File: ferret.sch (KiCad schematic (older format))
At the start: 0 parts

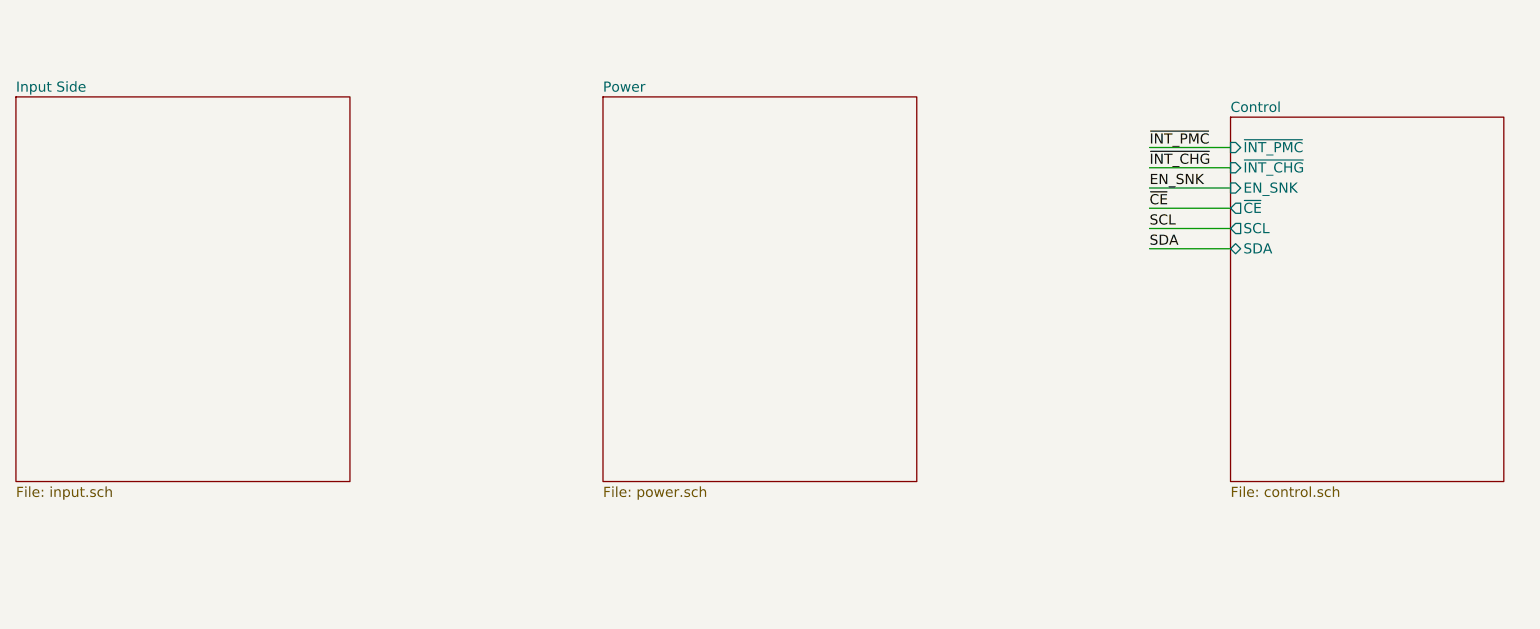
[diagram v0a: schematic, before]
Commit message: I'm pretty happy with it now, will place tomorrow
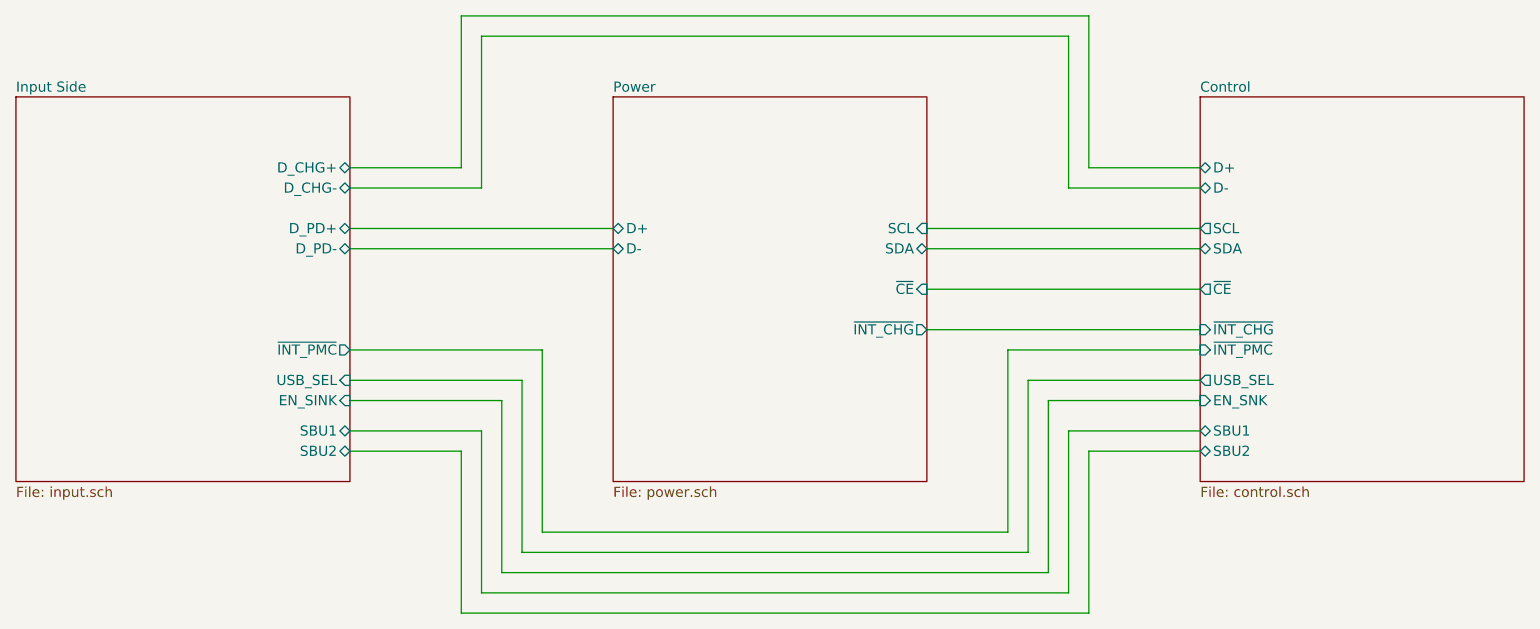
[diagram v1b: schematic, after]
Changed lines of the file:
@@
 Comment4 ""
 $EndDescr
-Text Label 7300 3050 0    50   ~ 0
-~CE
-Text Label 7300 3250 0    50   ~ 0
-SDA
-Text Label 7300 3150 0    50   ~ 0
-SCL
-Text Label 7300 2850 0    50   ~ 0
-~INT_CHG
-Text Label 7300 2750 0    50   ~ 0
-~INT_PMC
-Text Label 7300 2950 0    50   ~ 0
-EN_SNK
-Wire Wire Line
-	7300 2750 7700 2750
-Wire Wire Line
-	7700 2850 7300 2850
-Wire Wire Line
-	7300 2950 7700 2950
-Wire Wire Line
-	7700 3050 7300 3050
-Wire Wire Line
-	7700 3150 7300 3150
-Wire Wire Line
-	7300 3250 7700 3250
 $Sheet
 S 1700 2500 1650 1900
@@
 F0 "Input Side" 50
 F1 "input.sch" 50
+F2 "D_PD+" B R 3350 3150 50
+F3 "D_PD-" B R 3350 3250 50
+F4 "USB_SEL" I R 3350 3900 50
+F5 "D_CHG+" B R 3350 2850 50
+F6 "D_CHG-" B R 3350 2950 50
+F7 "SBU2" B R 3350 4250 50
+F8 "SBU1" B R 3350 4150 50
+F9 "~INT_PMC" O R 3350 3750 50
+F10 "EN_SINK" I R 3350 4000 50
 $EndSheet
 $Sheet
-S 4600 2500 1550 1900
+S 4650 2500 1550 1900
 U 5F165A7A
 F0 "Power" 50
 F1 "power.sch" 50
+F2 "D+" B L 4650 3150 50
+F3 "D-" B L 4650 3250 50
+F4 "~INT_CHG" O R 6200 3650 50
+F5 "SCL" I R 6200 3150 50
+F6 "SDA" B R 6200 3250 50
+F7 "~CE" I R 6200 3450 50
 $EndSheet
 $Sheet
-S 7700 2600 1350 1800
+S 7550 2500 1600 1900
 U 5EF44CB5
 F0 "Control" 50
 F1 "control.sch" 50
-F2 "~INT_PMC" I L 7700 2750 50
-F3 "EN_SNK" I L 7700 2950 50
-F4 "~CE" O L 7700 3050 50
-F5 "SCL" O L 7700 3150 50
-F6 "SDA" B L 7700 3250 50
-F7 "~INT_CHG" I L 7700 2850 50
+F2 "~INT_PMC" I L 7550 3750 50
+F3 "EN_SNK" I L 7550 4000 50
+F4 "~CE" O L 7550 3450 50
+F5 "SCL" O L 7550 3150 50
+F6 "SDA" B L 7550 3250 50
+F7 "~INT_CHG" I L 7550 3650 50
+F8 "D-" B L 7550 2950 50
+F9 "D+" B L 7550 2850 50
+F10 "SBU1" B L 7550 4150 50
+F11 "SBU2" B L 7550 4250 50
+F12 "USB_SEL" O L 7550 3900 50
 $EndSheet
+Wire Wire Line
+	6200 3250 7550 3250
+Wire Wire Line
+	7550 3150 6200 3150
+Wire Wire Line
+	7550 3450 6200 3450
+Wire Wire Line
+	3350 3150 4650 3150
+Wire Wire Line
+	4650 3250 3350 3250
+Wire Wire Line
+	6200 3650 7550 3650
+Wire Wire Line
+	3350 2850 3900 2850
+Wire Wire Line
+	3900 2850 3900 2100
+Wire Wire Line
+	3900 2100 7000 2100
+Wire Wire Line
+	7000 2100 7000 2850
+Wire Wire Line
+	7000 2850 7550 2850
+Wire Wire Line
+	3350 2950 4000 2950
+Wire Wire Line
+	4000 2950 4000 2200
+Wire Wire Line
+	4000 2200 6900 2200
+Wire Wire Line
+	6900 2200 6900 2950
+Wire Wire Line
+	6900 2950 7550 2950
+Wire Wire Line
+	3350 4250 3900 4250
+Wire Wire Line
+	3900 4250 3900 5050
+Wire Wire Line
+	3900 5050 7000 5050
+Wire Wire Line
+	7000 5050 7000 4250
+Wire Wire Line
+	7000 4250 7550 4250
+Wire Wire Line
+	7550 4150 6900 4150
+Wire Wire Line
+	6900 4150 6900 4950
+Wire Wire Line
+	6900 4950 4000 4950
+Wire Wire Line
+	4000 4950 4000 4150
+Wire Wire Line
+	4000 4150 3350 4150
+Wire Wire Line
+	3350 4000 4100 4000
+Wire Wire Line
+	4100 4000 4100 4850
+Wire Wire Line
+	4100 4850 6800 4850
+Wire Wire Line
+	6800 4850 6800 4000
+Wire Wire Line
+	6800 4000 7550 4000
+Wire Wire Line
+	3350 3900 4200 3900
+Wire Wire Line
+	4200 3900 4200 4750
+Wire Wire Line
+	4200 4750 6700 4750
+Wire Wire Line
+	6700 4750 6700 3900
+Wire Wire Line
+	6700 3900 7550 3900
+Wire Wire Line
+	7550 3750 6600 3750
+Wire Wire Line
+	6600 3750 6600 4650
+Wire Wire Line
+	6600 4650 4300 4650
+Wire Wire Line
+	4300 4650 4300 3750
+Wire Wire Line
+	4300 3750 3350 3750
 $EndSCHEMATC
